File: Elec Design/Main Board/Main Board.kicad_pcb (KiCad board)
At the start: 2 copper layers, 47.2 x 115.3 mm, 27 parts, among them J1 302-S101, J2 LPC1768 Socket, J3 PJ-102A, J4 OSTTC020162, J5 OSTTC030162, J6 0022232041, U2 MCP2551-I-P, U3 NCP718xSN500, U4 NCP718xSN330

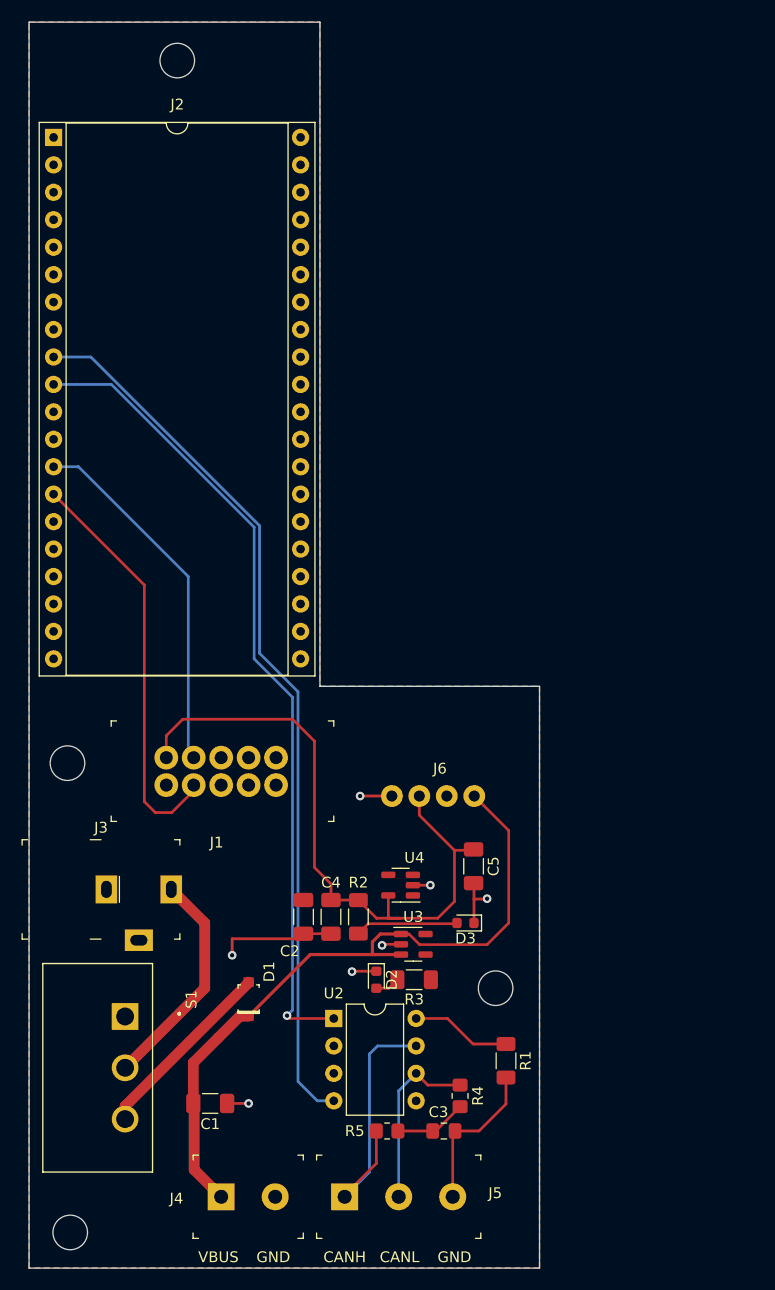
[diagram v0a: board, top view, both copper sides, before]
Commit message: converting to git structure
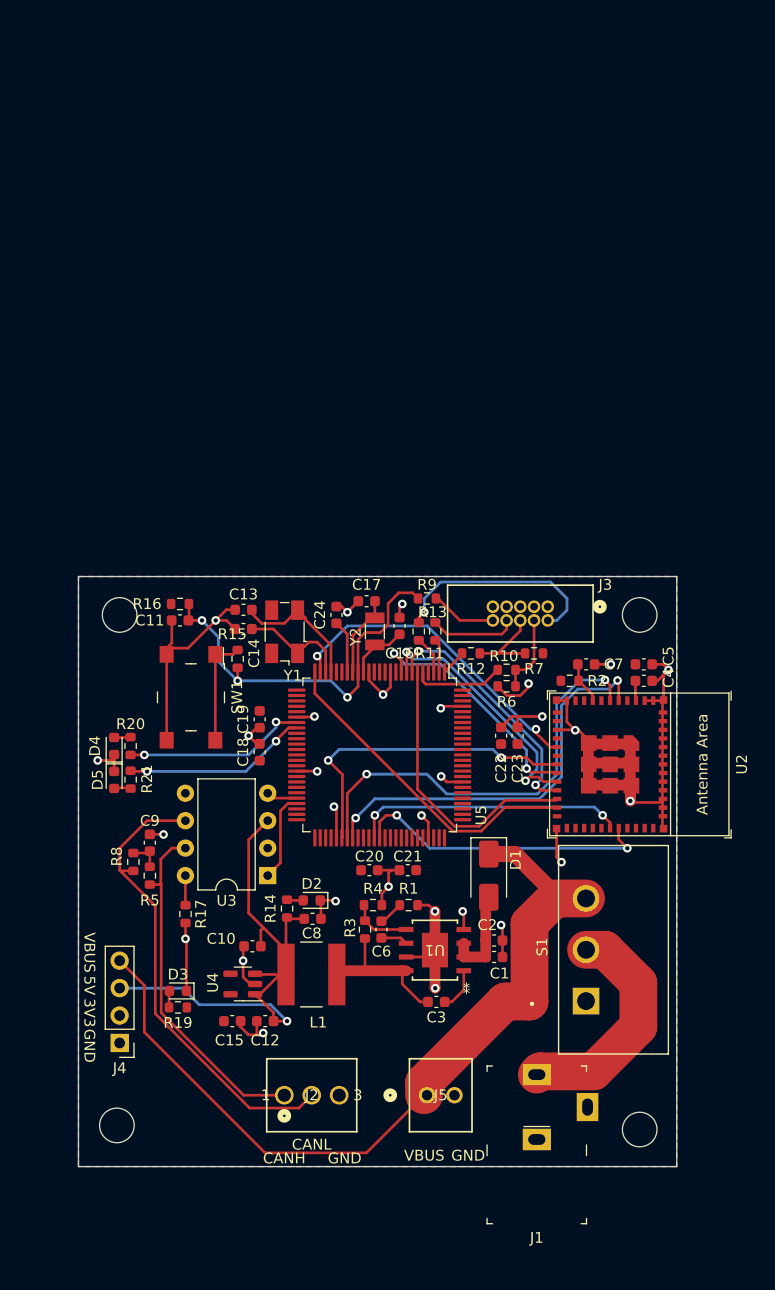
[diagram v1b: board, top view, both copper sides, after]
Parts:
- removed J6: 0022232041, digikey-footprints:PinHeader_1x4_P2.54mm_Drill1.02mm
- removed the REF** at (100.1, 27.4)
- removed the REF** at (129.5, 113.3)
- removed the REF** at (89.9, 92.5)
- removed the REF** at (90.2, 135.9)
- added C10: 22uF, Capacitor_SMD:C_0603_1608Metric, F.Cu at (107.0, 109.4)
- added C11: 100nF, Capacitor_SMD:C_0603_1608Metric, F.Cu at (100.3, 79.2)
- added C12: 1uF, Capacitor_SMD:C_0603_1608Metric, F.Cu at (108.2, 116.3)
- added C13: 18pF, Capacitor_SMD:C_0603_1608Metric, F.Cu at (106.2, 78.3)
- added C14: 18pF, Capacitor_SMD:C_0603_1608Metric, F.Cu at (106.2, 80.0)
- added C15: 1uF, Capacitor_SMD:C_0603_1608Metric, F.Cu at (105.2, 116.3)
- added C16: 18pF, Capacitor_SMD:C_0603_1608Metric, F.Cu at (120.7, 79.8)
- added C17: 18pF, Capacitor_SMD:C_0603_1608Metric, F.Cu at (117.6, 77.5)
- added C18: 100nF, Capacitor_SMD:C_0603_1608Metric, F.Cu at (107.7, 91.4)
- added C19: 10nF, Capacitor_SMD:C_0603_1608Metric, F.Cu at (107.7, 88.4)
- added C20: 100nF, Capacitor_SMD:C_0603_1608Metric, F.Cu at (117.9, 102.4)
- added C21: 10nF, Capacitor_SMD:C_0603_1608Metric, F.Cu at (121.4, 102.4)
- added C22: 100nF, Capacitor_SMD:C_0603_1608Metric, F.Cu at (130.0, 89.9)
- added C23: 10nF, Capacitor_SMD:C_0603_1608Metric, F.Cu at (131.6, 89.9)
- added C24: 100nF, Capacitor_SMD:C_0603_1608Metric, F.Cu at (114.8, 78.7)
- added C6: 6800pF, Capacitor_SMD:C_0603_1608Metric, F.Cu at (119.0, 107.9)
- added C7: 1uF, Capacitor_SMD:C_0603_1608Metric, F.Cu at (137.9, 83.3)
- added C8: 22uF, Capacitor_SMD:C_0603_1608Metric, F.Cu at (112.6, 106.9)
- added C9: 1nF, Capacitor_SMD:C_0603_1608Metric, F.Cu at (97.5, 99.8)
- added D4: LED Low current, LED_SMD:LED_0603_1608Metric, F.Cu at (94.2, 90.9)
- added D5: LED Low current, LED_SMD:LED_0603_1608Metric, F.Cu at (94.2, 94.0)
- added L1: 4.7uH, NR6028T4R7M:IND_NR6028T4R7M, F.Cu at (112.5, 112.0)
- added R10: 50R, Resistor_SMD:R_0603_1608Metric, F.Cu at (130.6, 83.8)
- added R11: 50R, Resistor_SMD:R_0603_1608Metric, F.Cu at (122.4, 80.3)
- added R12: 50R, Resistor_SMD:R_0603_1608Metric, F.Cu at (127.3, 82.3)
- added R13: 50R, Resistor_SMD:R_0603_1608Metric, F.Cu at (124.0, 80.3)
- added R14: 1k6, Resistor_SMD:R_0603_1608Metric, F.Cu at (110.2, 105.9)
- added R15: 100R, Resistor_SMD:R_0603_1608Metric, F.Cu at (105.7, 82.8)
- added R16: 100k, Resistor_SMD:R_0603_1608Metric, F.Cu at (100.3, 77.7)
- added R17: 10k, Resistor_SMD:R_0603_1608Metric, F.Cu at (100.8, 106.4)
- added R19: 750R, Resistor_SMD:R_0603_1608Metric, F.Cu at (100.1, 115.1)
- added R20: 750R, Resistor_SMD:R_0603_1608Metric, F.Cu at (95.8, 90.9)
- added R21: 750R, Resistor_SMD:R_0603_1608Metric, F.Cu at (95.8, 94.0)
- added R6: 10k, Resistor_SMD:R_0603_1608Metric, F.Cu at (130.6, 85.3)
- added R7: 10k, Resistor_SMD:R_0603_1608Metric, F.Cu at (133.1, 82.3)
- added R8: 60R, Resistor_SMD:R_0603_1608Metric, F.Cu at (96.0, 101.6)
- added R9: 50R, Resistor_SMD:R_0603_1608Metric, F.Cu at (123.2, 77.2)
- added REF**: MountingHole_3.2mm_M3, MountingHole:MountingHole_3.2mm_M3, F.Cu at (142.9, 126.4)
- added REF**: MountingHole_3.2mm_M3, MountingHole:MountingHole_3.2mm_M3, F.Cu at (142.9, 78.7)
- added REF**: MountingHole_3.2mm_M3, MountingHole:MountingHole_3.2mm_M3, F.Cu at (94.7, 78.7)
- added REF**: MountingHole_3.2mm_M3, MountingHole:MountingHole_3.2mm_M3, F.Cu at (94.5, 126.0)
- added SW1: SW_SPST, digikey-footprints:Switch_Tactile_SMD_6x6mm_PTS645, F.Cu at (101.3, 86.4)
- added U1: BD9E302EFJ-E2, BD9E302EFJ-E2:HTSOP-J8_ROM, F.Cu at (123.9, 109.8)
- added U5: LPC1768FBD100, Package_QFP:LQFP-100_14x14mm_P0.5mm, F.Cu at (118.8, 91.7)
- added Y1: 12MHz/10pF, Crystal:Crystal_SMD_Abracon_ABM3B-4Pin_5.0x3.2mm, F.Cu at (110.0, 80.3)
- added Y2: 32.768kHz/9pF, Crystal:Crystal_SMD_3215-2Pin_3.2x1.5mm, F.Cu at (118.4, 80.3)
- C1, C4: footprint Capacitor_SMD:C_1206_3216Metric_Pad1.33x1.80mm_HandSolder -> Capacitor_SMD:C_0603_1608Metric
- C2: value 10uF -> 0.1uF; footprint Capacitor_SMD:C_1206_3216Metric_Pad1.33x1.80mm_HandSolder -> Capacitor_SMD:C_0603_1608Metric
- C3: value 1nF -> 0.1uF; footprint Capacitor_SMD:C_0805_2012Metric_Pad1.18x1.45mm_HandSolder -> Capacitor_SMD:C_0603_1608Metric
- C5: value 100nF -> 0.1uF; footprint Capacitor_SMD:C_1206_3216Metric_Pad1.33x1.80mm_HandSolder -> Capacitor_SMD:C_0603_1608Metric
- D1: value 1N5819HW-7-F -> B340; footprint digikey-footprints:SOD-123 -> Diode_SMD:D_SMA
- J1: value 302-S101 -> PJ-102A; footprint digikey-footprints:PinHeader_2x5_P2.54mm_Drill1.2mm -> digikey-footprints:Barrel_Jack_5.5mmODx2.1mmID_PJ-102A
- J2: value LPC1768 Socket -> ~; footprint Package_DIP:DIP-40_W22.86_Socket -> 1x3 terminal block:CONN_282834-3_TYC
- J3: value PJ-102A -> Conn_ARM_JTAG_SWD_10; footprint digikey-footprints:Barrel_Jack_5.5mmODx2.1mmID_PJ-102A -> 10 pin jtag:CONN_3220-10-0100-00_CNC
- J4: value OSTTC020162 -> 0022232041; footprint digikey-footprints:Term_Block_1x2_P5mm -> Connector_PinHeader_2.54mm:PinHeader_1x04_P2.54mm_Vertical
- J5: value OSTTC030162 -> ~; footprint digikey-footprints:Term_Block_1x3_P5mm -> 1x2 terminal block:CONN2_282834-2_TEC
- R1: footprint Resistor_SMD:R_1206_3216Metric_Pad1.30x1.75mm_HandSolder -> Resistor_SMD:R_0603_1608Metric
- R2: value 750R -> 10k; footprint Resistor_SMD:R_1206_3216Metric_Pad1.30x1.75mm_HandSolder -> Resistor_SMD:R_0603_1608Metric
- R3: value 1k6 -> 430k; footprint Resistor_SMD:R_1206_3216Metric_Pad1.30x1.75mm_HandSolder -> Resistor_SMD:R_0603_1608Metric
- R4: value 60R -> 82k; footprint Resistor_SMD:R_0805_2012Metric_Pad1.20x1.40mm_HandSolder -> Resistor_SMD:R_0603_1608Metric
- R5: footprint Resistor_SMD:R_0805_2012Metric_Pad1.20x1.40mm_HandSolder -> Resistor_SMD:R_0603_1608Metric
- U2: value MCP2551-I-P -> ESP32-C3-MINI-1; footprint Package_DIP:DIP-8_W7.62mm -> Espressif:ESP32-C3-MINI-1
- U3: value NCP718xSN500 -> MCP2551-I-P; footprint Package_TO_SOT_SMD:SOT-23-5 -> Package_DIP:DIP-8_W7.62mm
- moved J2 66.5 mm to (110.0, 123.2)
- moved J1 47.1 mm to (133.3, 124.3), turned to 180 degrees
- moved J3 46.0 mm to (134.4, 78.0), turned to 180 degrees
- moved S1 44.0 mm to (137.9, 109.7), turned to 90 degrees
- moved U2 36.8 mm to (142.8, 92.6), turned to -90 degrees
- moved C4 36.3 mm to (143.3, 84.8), turned to 0 degrees
- moved R5 32.3 mm to (97.5, 102.9), turned to 90 degrees
- moved C1 29.6 mm to (129.4, 110.4)
- moved R2 29.3 mm to (136.4, 84.8), turned to 180 degrees
- moved D3 27.3 mm to (100.1, 113.5)
- moved D1 25.0 mm to (128.9, 102.9), turned to -90 degrees
- moved C5 24.4 mm to (143.3, 83.3), turned to 0 degrees
- moved R4 19.4 mm to (118.2, 105.6), turned to 0 degrees
- moved C2 17.8 mm to (129.4, 108.9), turned to 0 degrees
- moved U4 17.2 mm to (106.1, 112.9)
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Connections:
- C1 pad 1: VBUS -> Net-(D1-A)
- C2 pad 1: +5V -> Net-(D1-A)
- C3 pad 1: Net-(C3-Pad1) -> Net-(U1-BOOT)
- C3 pad 2: GND -> Net-(U1-SW)
- D2 pad 2: Net-(D2-Pad2) -> Net-(D2-A)
- D3 pad 2: Net-(R2-Pad2) -> Net-(D3-A)
- J1 pad 1: +3.3V -> Net-(J1-Pad1)
- J1 pad 3: Net-(J1-Pad3) -> GND
- J2 pad 1: GND -> /CANH
- J2 pad 2: +5V -> /CANL
- J2 pad 3: unconnected-(J2-Pad3) -> GND
- J3 pad 1: Net-(J3-Pad1) -> +3.3V
- J3 pad 2: GND -> Net-(J3-SWDIO/TMS)
- J4 pad 1: VBUS -> GND
- J4 pad 2: GND -> +3.3V
- J5 pad 1: /CANH -> VBUS
- J5 pad 2: /CANL -> GND
- R1 pad 1: Net-(U2-Pad8) -> Net-(C6-Pad2)
- R2 pad 1: +3.3V -> Net-(U2-EN/CHIP_PU)
- R2 pad 2: Net-(R2-Pad2) -> +3.3V
- R3 pad 1: +5V -> Net-(U1-SW)
- R3 pad 2: Net-(D2-Pad2) -> Net-(U1-FB)
- R4 pad 1: /CANL -> Net-(U1-FB)
- R4 pad 2: Net-(C3-Pad1) -> GND
- R5 pad 2: Net-(C3-Pad1) -> Net-(C9-Pad1)
- S1 pad 2: Net-(J3-Pad1) -> Net-(J1-Pad1)
- S1 pad 3: Net-(D1-PadA) -> VBUS
- U2 pad 1: Net-(J2-Pad10) -> GND
- U2 pad 3: +5V -> +3.3V
- U2 pad 4: Net-(U2-Pad4) -> unconnected-(U2-NC-Pad4)
- U2 pad 5: unconnected-(U2-Pad5) -> Net-(U2-GPIO2/ADC1_CH2)
- U2 pad 6: /CANL -> Net-(U2-GPIO3/ADC1_CH3)
- U2 pad 7: /CANH -> unconnected-(U2-NC-Pad7)
- U2 pad 8: Net-(U2-Pad8) -> Net-(U2-EN/CHIP_PU)
- U3 pad 1: VBUS -> Net-(U3-TXD)
- U3 pad 3: VBUS -> +5V
- U3 pad 4: unconnected-(U3-Pad4) -> Net-(U3-RXD)
- U3 pad 5: +5V -> unconnected-(U3-Vref-Pad5)
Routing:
- net GND: track 41.4 -> 158.2 mm, vias 7 -> 29
- net Net-(U2-Pad4): track 82.5 -> 0.00 mm
- net Net-(J2-Pad10): track 75.4 -> 0.00 mm, vias 1 -> 0
- net +3.3V: track 61.4 -> 6.77 mm
- net +5V: track 0.00 -> 50.7 mm, vias 0 -> 1
- net Net-(U2-GPIO3/ADC1_CH3): track 0.00 -> 39.8 mm, vias 0 -> 2
- net Net-(J1-Pad4): track 38.3 -> 0.00 mm
- net Net-(U2-GPIO2/ADC1_CH2): track 0.00 -> 37.2 mm, vias 0 -> 2
- net /RESET: track 0.00 -> 36.1 mm, vias 0 -> 3
- net Net-(J1-Pad3): track 33.6 -> 0.00 mm
- net Net-(U2-GPIO9): track 0.00 -> 30.6 mm
- net Net-(U2-GPIO4/ADC1_CH4): track 0.00 -> 29.9 mm, vias 0 -> 2
- net Net-(U2-GPIO10): track 0.00 -> 29.8 mm, vias 0 -> 2
- net Net-(U2-GPIO21/U0TXD): track 0.00 -> 28.1 mm, vias 0 -> 2
- net /CANL: track 16.6 -> 44.2 mm
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- added copper zone on F.Cu, net +3.3V
- removed copper zone on F.Cu, net +5V
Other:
- board size 47.2 x 115.3 mm -> 55.4 x 54.6 mm
- board text added: "3V3"
- board text added: "5V"
